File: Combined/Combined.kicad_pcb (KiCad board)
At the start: 4 copper layers, 13 parts, among them U1 ATMEGA168PA-MU, U2 RA-08H(915), U3 ATGM336H-5N31, U4 X1B000301000200

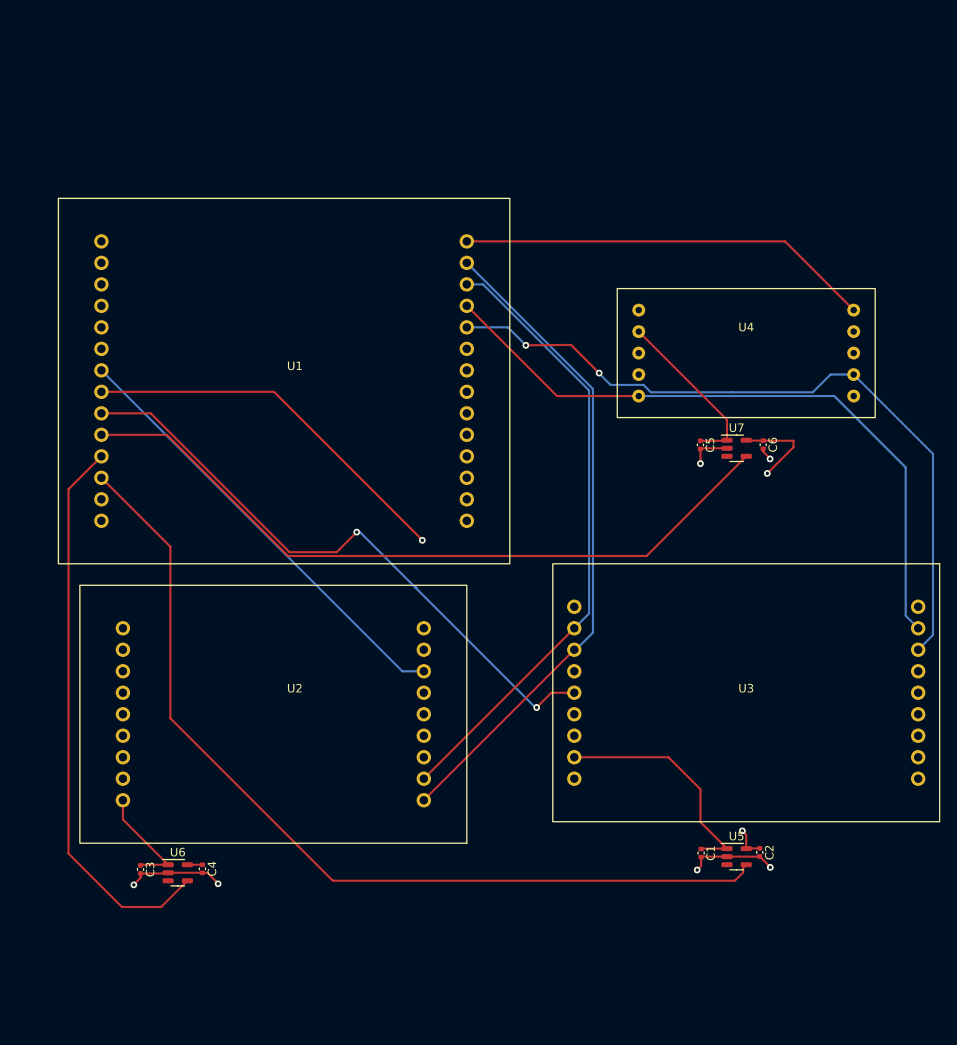
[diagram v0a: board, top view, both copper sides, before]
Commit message: Working.
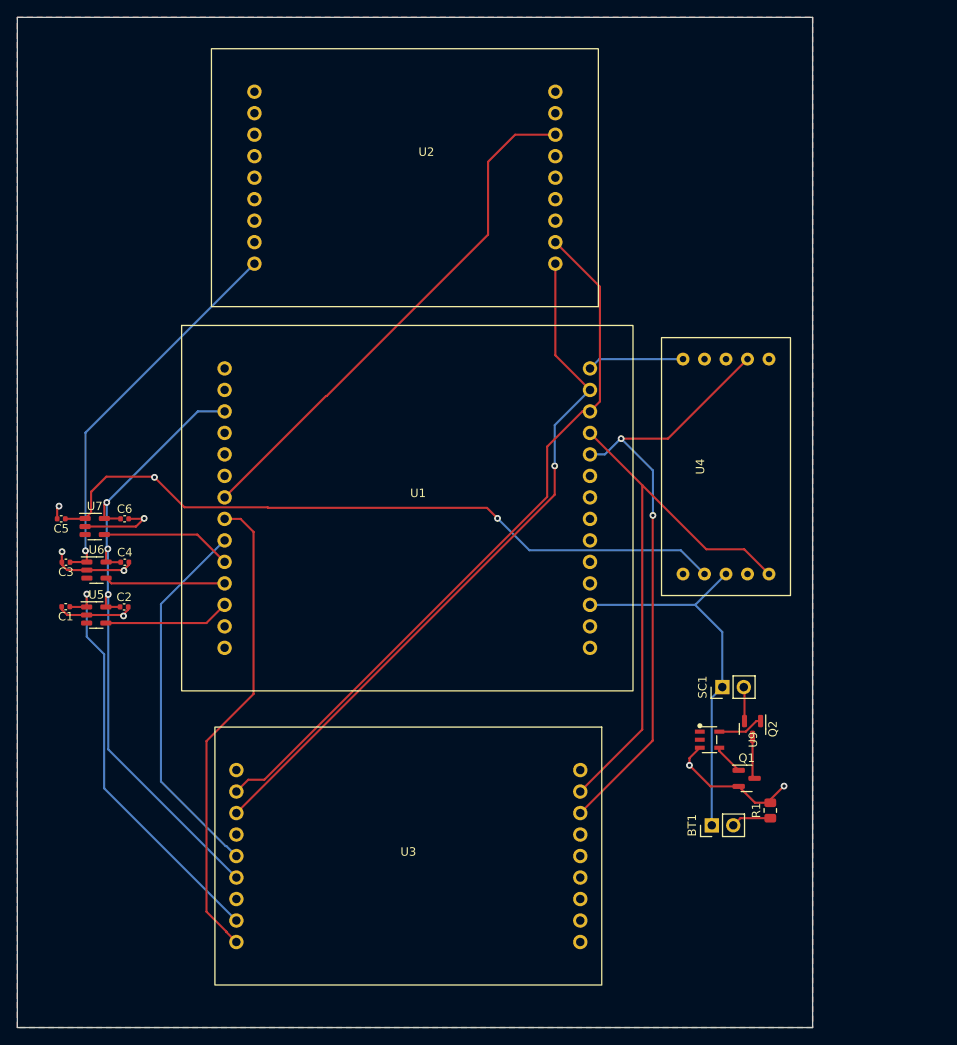
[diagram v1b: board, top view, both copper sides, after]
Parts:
- added BT1: RJD2048(Bat), Connector_PinHeader_2.54mm:PinHeader_1x02_P2.54mm_Vertical, F.Cu at (178.6, 138.7)
- added Q1: 2N7002E, Package_TO_SOT_SMD:SOT-23, F.Cu at (182.7, 133.1)
- added Q2: 2N7002E, Package_TO_SOT_SMD:SOT-23, F.Cu at (183.4, 127.3)
- added R1: 0.01, Resistor_SMD:R_0805_2012Metric, F.Cu at (185.5, 136.9)
- added SC1: KXOB081K06TF-TR, Connector_PinHeader_2.54mm:PinHeader_1x02_P2.54mm_Vertical, F.Cu at (179.8, 122.3)
- added U9: AP9101CK-AHTRG1, PARTS:SOT-23-5_L3.0-W1.7-P0.95-LS2.8-BL, F.Cu at (178.3, 128.5)
- moved U5 80.9 mm to (105.8, 113.8)
- moved C1 80.5 mm to (102.2, 112.8), turned to 180 degrees
- moved C2 80.5 mm to (109.1, 112.9), turned to 0 degrees
- moved U7 76.4 mm to (105.7, 103.4)
- moved C5 76.0 mm to (101.7, 102.4), turned to 180 degrees
- moved C6 76.0 mm to (109.2, 102.4), turned to 0 degrees
- moved U2 65.3 mm to (144.9, 59.6)
- moved U3 44.4 mm to (142.7, 142.3)
- moved C4 37.4 mm to (109.2, 107.6), turned to 0 degrees
- moved C3 37.4 mm to (102.3, 107.6), turned to 180 degrees
- moved U6 37.0 mm to (105.9, 108.5)
- moved U1 20.9 mm to (143.9, 99.9)
- moved U4 14.2 mm to (179.8, 96.3), turned to 90 degrees
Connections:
- U1 pad 19: /VBAT -> VCC
- U1 pad 22: unconnected-(U1-ADC7-Pad22) -> /VBAT_SNS
- U3 pad 6: /VBAT -> VCC
- U4 pad 3: /VBAT -> VCC
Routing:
- net /GPS_EN: track 108.9 -> 14.9 mm
- net /RTC_EN: track 87.0 -> 15.5 mm
- net /RTC_VCC: track 20.3 -> 84.0 mm, vias 0 -> 2
- net /LORA_EN: track 66.5 -> 14.3 mm
- net /VBAT_SNS: track 0.00 -> 42.9 mm
- net /RTC_INT: track 49.1 -> 11.4 mm
- net /LORA_VCC: track 13.1 -> 45.6 mm, vias 0 -> 1
- net /GPS_I/O: track 73.2 -> 44.2 mm, vias 2 -> 0
- net VCC: track 204.7 -> 178.0 mm, vias 2 -> 3
- net /GPS_RESET: track 80.9 -> 56.3 mm, vias 1 -> 0
- net /GPS_VCC: track 27.9 -> 49.4 mm, vias 0 -> 1
- net GND: track 28.7 -> 48.1 mm, vias 6 -> 7
- net /SDA: track 87.0 -> 72.8 mm
- net /TX: track 73.6 -> 86.5 mm
- net /SCL: track 79.4 -> 67.3 mm
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- added copper zone on B.Cu, net GND
- added copper zone on F.Cu, net GND
- added copper zone on In1.Cu, net GND
- added copper zone on In2.Cu, net GND
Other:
- board outline added: 94 x 119.4 mm
